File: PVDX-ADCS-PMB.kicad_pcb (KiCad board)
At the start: 4 copper layers, 82.5 x 82.5 mm, 114 parts, among them J1 Conn_02x18_Row_Letter_Last, J2 Conn_01x18, J3 Conn_01x06, J4 Conn_01x02, J5 Conn_01x17, J6 Conn_01x03, J7 Conn_01x09, U1 TLV9001IDCK, U10 DRV8837C, U11 OPA2381AIDGKR, U12 OPA2381AIDGKR, U13 OPA2381AIDGKR, U14 OPA2381AIDGKR, U15 OPA2381AIDGKR, U16 OPA2381AIDGKR, U17 OPA2381AIDGKR, U18 OPA2381AIDGKR, U19 OPA2381AIDGKR, U2 INA226, U3 DRV8837C, U4 DRV8837C, U5 MCP23017x-x-SO, U6 ADG734BRUZ, U7 ADG734BRUZ, U8 ADG734BRUZ, U9 ADG734BRUZ

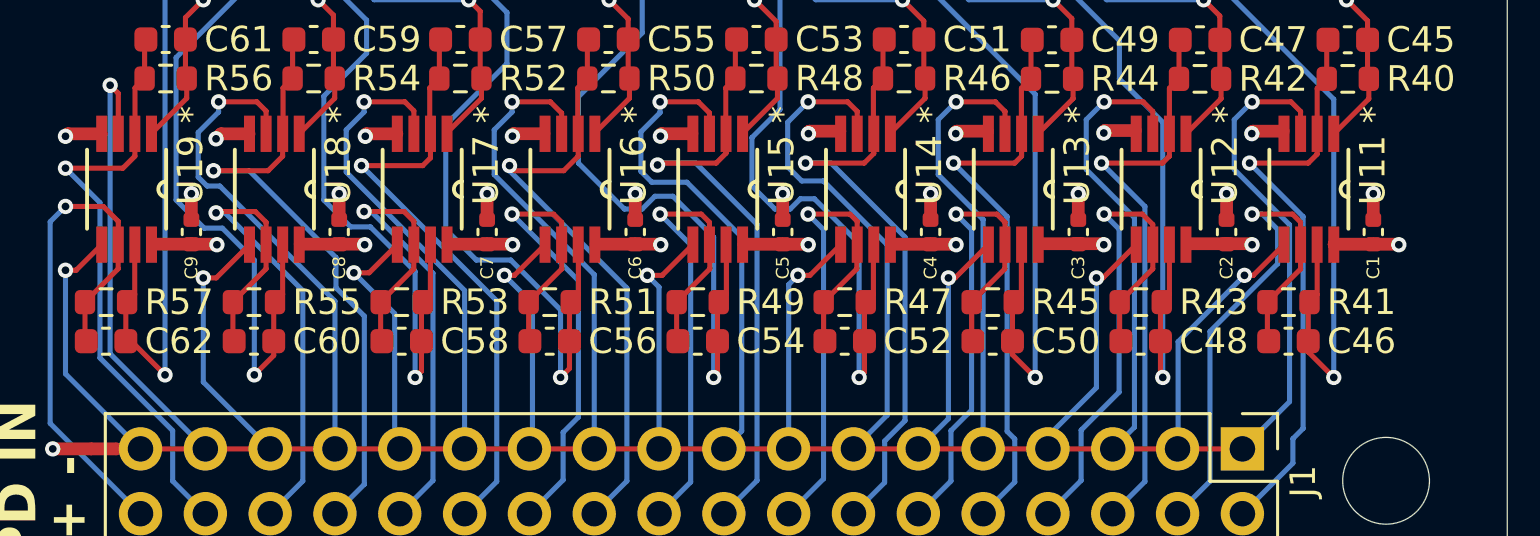
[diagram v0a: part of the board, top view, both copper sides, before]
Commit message: fix silkscreen, regen STEP, fix for ERC/DRC
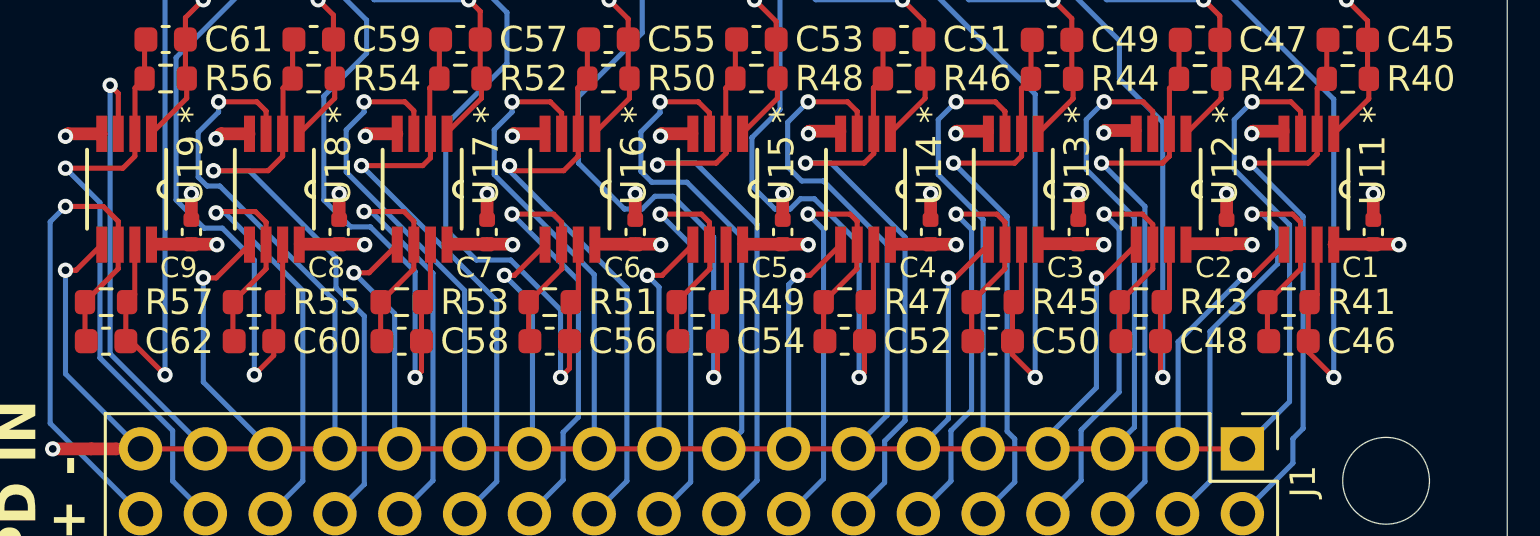
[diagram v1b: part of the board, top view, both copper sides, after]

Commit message: Prepared for fab: generated gerbers, switched PD C_fb from 22pF to 150pF, generated BOM, updated readme
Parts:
- C45, C46, C47, C48, C49, C50, C51, C52, C53, C54, C55, C56, C57, C58, C59, C60, C61, C62: value 22p -> 150p
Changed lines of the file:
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@@
 		(capping no)
 		(filling no)
+		(zone_defaults)
 		(grid_origin 140 120)
 		(pcbplotparams
@@
 			(plot_on_all_layers_selection 0x00000000_00000000_00000000_00000000)
 			(disableapertmacros no)
-			(usegerberextensions no)
+			(usegerberextensions yes)
 			(usegerberattributes yes)
 			(usegerberadvancedattributes yes)
@@
 			(outputformat 1)
 			(mirror no)
-			(drillshape 1)
+			(drillshape 0)
 			(scaleselection 1)
-			(outputdirectory "")
+			(outputdirectory "manufacturing/rev-1.1_2026-09-04/gerbers/")
 		)
 	)
@@
 			)
 		)
-		(property "Value" "22p"
+		(property "Value" "150p"
 			(at 0 1.43 0)
 			(layer "F.Fab")
@@
 			)
 		)
-		(property "Value" "22p"
+		(property "Value" "150p"
 			(at 0 1.43 0)
 			(layer "F.Fab")
@@
 			)
 		)
-		(property "Value" "22p"
+		(property "Value" "150p"
 			(at 0 1.43 0)
 			(layer "F.Fab")
@@
 			)
 		)
-		(property "Value" "22p"
+		(property "Value" "150p"
 			(at 0 1.43 0)
 			(layer "F.Fab")
@@
 			)
 		)
-		(property "Value" "22p"
+		(property "Value" "150p"
 			(at 0 1.43 0)
 			(layer "F.Fab")
@@
 			)
 		)
-		(property "Value" "22p"
+		(property "Value" "150p"
 			(at 0 1.43 0)
 			(layer "F.Fab")
@@
 			)
 		)
-		(property "Value" "22p"
+		(property "Value" "150p"
 			(at 0 1.43 0)
 			(layer "F.Fab")
@@
 			)
 		)
-		(property "Value" "22p"
+		(property "Value" "150p"
 			(at 0 1.43 0)
 			(layer "F.Fab")
@@
 			)
 		)
-		(property "Value" "22p"
+		(property "Value" "150p"
 			(at 0 1.43 0)
 			(layer "F.Fab")
@@
 			)
 		)
-		(property "Value" "22p"
+		(property "Value" "150p"
 			(at 0 1.43 0)
 			(layer "F.Fab")
@@
 			)
 		)
-		(property "Value" "22p"
+		(property "Value" "150p"
 			(at 0 1.43 0)
 			(layer "F.Fab")
@@
 			)
 		)
-		(property "Value" "22p"
+		(property "Value" "150p"
 			(at 0 1.43 0)
 			(layer "F.Fab")
@@
 			)
 		)
-		(property "Value" "22p"
+		(property "Value" "150p"
 			(at 0 1.43 0)
 			(layer "F.Fab")
@@
 			)
 		)
-		(property "Value" "22p"
+		(property "Value" "150p"
 			(at 0 1.43 0)
 			(layer "F.Fab")
@@
 			)
 		)
-		(property "Value" "22p"
+		(property "Value" "150p"
 			(at 0 1.43 0)
 			(layer "F.Fab")
@@
 			)
 		)
-		(property "Value" "22p"
+		(property "Value" "150p"
 			(at 0 1.43 0)
 			(layer "F.Fab")
@@
 			)
 		)
-		(property "Value" "22p"
+		(property "Value" "150p"
 			(at 0 1.43 0)
 			(layer "F.Fab")
@@
 			)
 		)
-		(property "Value" "22p"
+		(property "Value" "150p"
 			(at 0 1.43 0)
 			(layer "F.Fab")
